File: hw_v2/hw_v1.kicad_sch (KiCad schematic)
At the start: 54 parts, among them J16 47352-1001, J8 USB_B, J9 Tag connect, SW1 SW_Push, SW2 SW_Push, U13 STM32F407VGTx, U14 TJA1051T-3, U15 25Q16, U16 REF3033, U17 SRV05-4, Y1 32.768kHz, Y2 25MHz

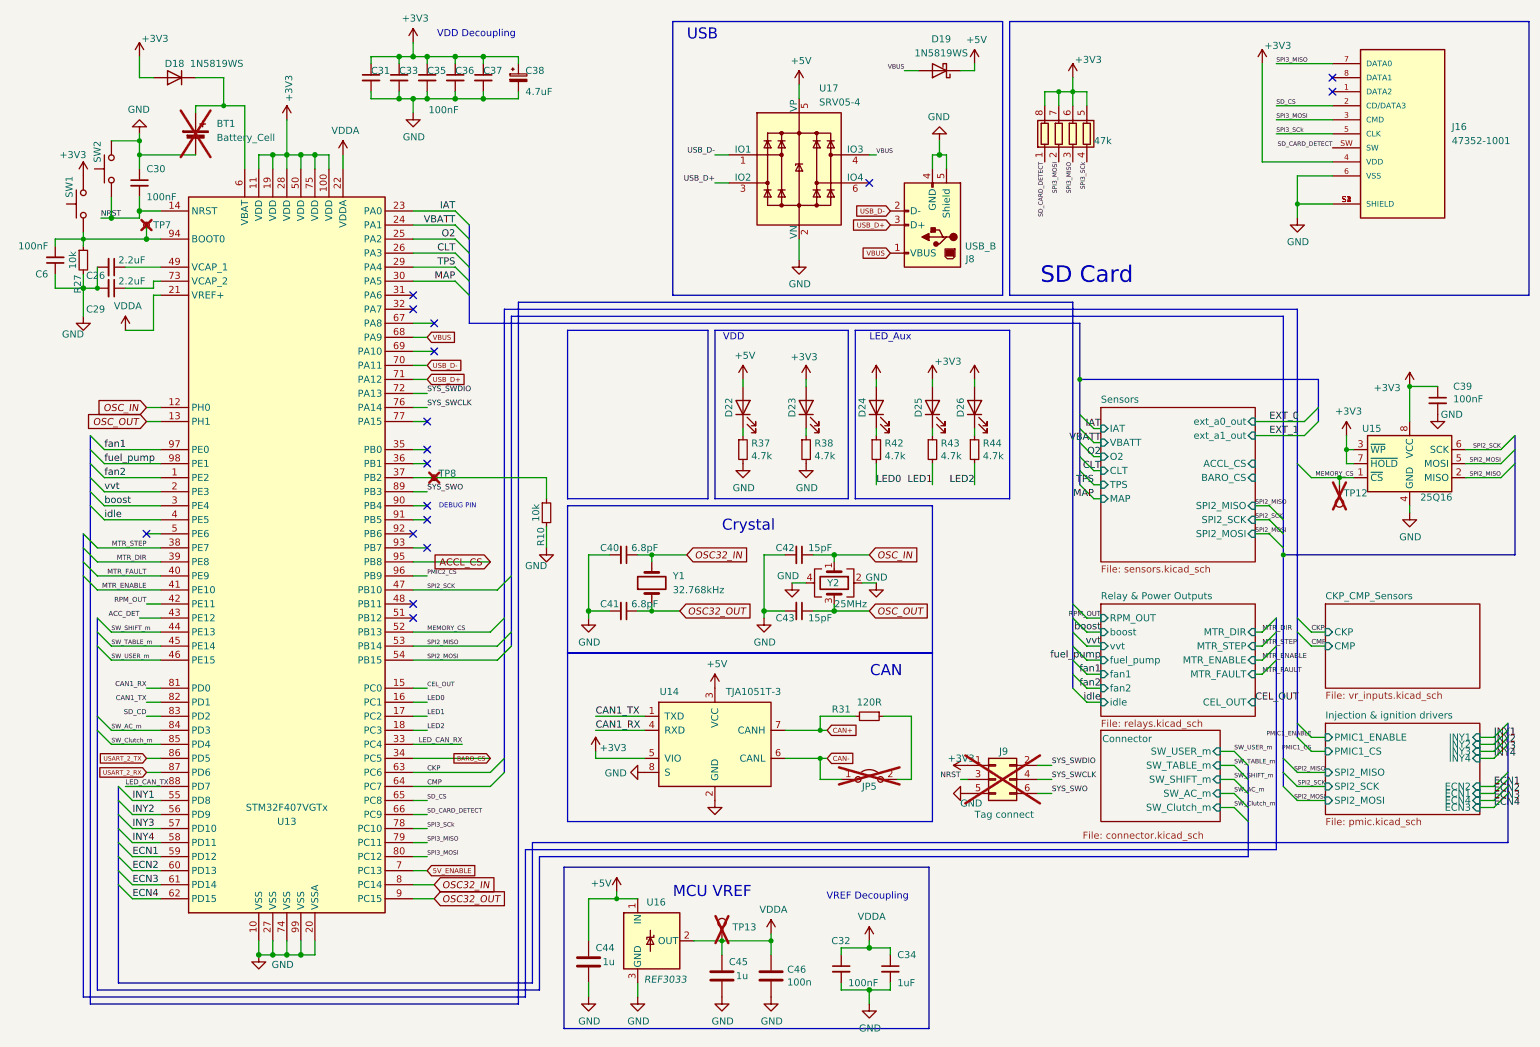
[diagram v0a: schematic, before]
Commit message: planito mas catolico
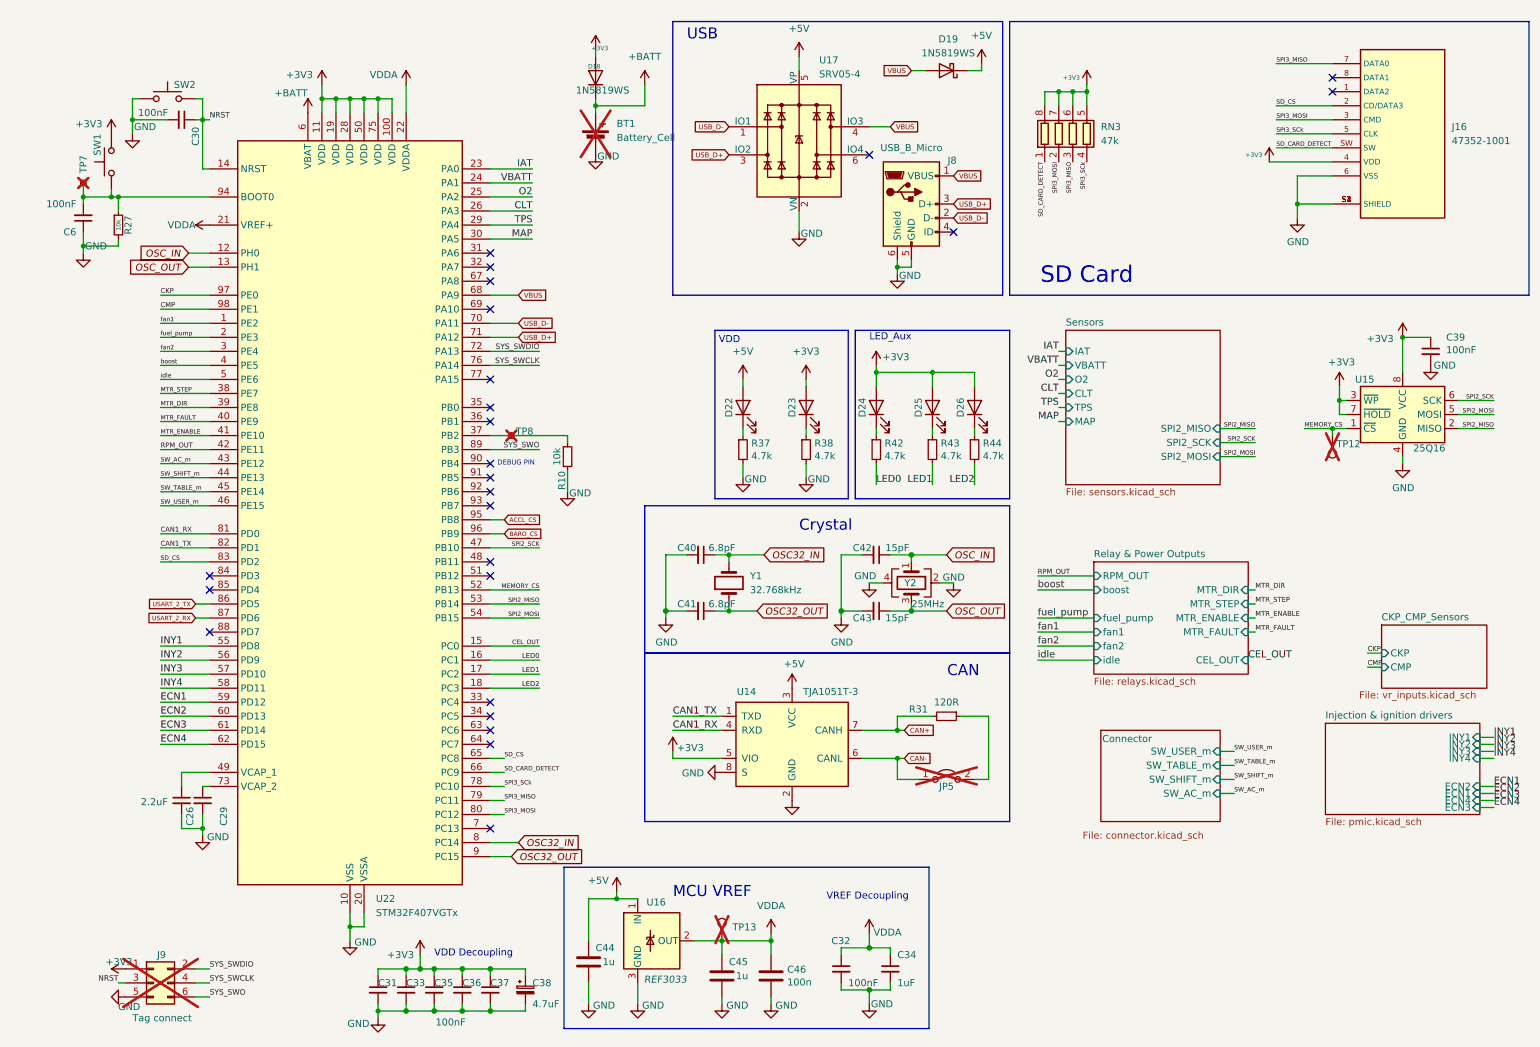
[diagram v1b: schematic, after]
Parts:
- removed J8: USB_B, Connector_USB:USB_Mini-B_Tensility_54-00023_Vertical, symbol STM32F_rev3-rescue:USB_B-Connector
- removed U13: STM32F407VGTx, Package_QFP:LQFP-100_14x14mm_P0.5mm, symbol MCU_ST_STM32F4:STM32F407VGTx
- added J8: USB_B_Micro, Connector_USB:USB_Mini-B_Tensility_54-00023_Vertical, symbol Connector:USB_B_Micro
- added U22: STM32F407VGTx, Package_QFP:LQFP-100_14x14mm_P0.5mm, symbol MCU_ST_STM32F4:STM32F407VGTx
- D18: footprint Diode_SMD:D_SOD-323_HandSoldering -> Diode_SMD:D_SOD-323
- J16: footprint uEFI_v5:MOLEX_47352-1001 -> hw_v2lib:47352-1001; symbol uEFI_v5:47352-1001 -> hw_v2:47352-1001
- RN3: footprint Resistor_SMD:R_Array_Convex_4x0603 -> (none); LCSC C779384 -> (none)
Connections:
- net +3V3: now also U22.100 (VDD), U22.11 (VDD), U22.19 (VDD), U22.28 (VDD), U22.50 (VDD), U22.75 (VDD)
- net ACCL_CS: now also U22.95 (PB8)
- net BARO_CS: now also U22.96 (PB9)
- net CAN1_RX: now also U22.81 (PD0)
- net CAN1_TX: now also U22.82 (PD1)
- net CEL_OUT: now also U22.15 (PC0)
- net CKP: now also U22.97 (PE0)
- net CLT: now also U22.26 (PA3)
- net CMP: now also U22.98 (PE1)
- net ECN1: now also U22.59 (PD12)
- net ECN2: now also U22.60 (PD13)
- net ECN3: now also U22.61 (PD14)
- net ECN4: now also U22.62 (PD15)
- net GND: now also C30.2, SW2.1, J8.5 (GND), J8.6 (Shield), U22.10 (VSS), U22.20 (VSSA), U22.27 (VSS), U22.74 (VSS), U22.99 (VSS); no longer C30.1, SW2.2
- net IAT: now also U22.23 (PA0)
- net INY1: now also U22.55 (PD8)
- net INY2: now also U22.56 (PD9)
- net INY3: now also U22.57 (PD10)
- net INY4: now also U22.58 (PD11)
- net LED0: now also U22.16 (PC1)
- net LED1: now also U22.17 (PC2)
- net LED2: now also U22.18 (PC3)
- net MAP: now also U22.30 (PA5)
- net MEMORY_CS: now also U22.52 (PB13)
- net MTR_DIR: now also U22.39 (PE8)
- net MTR_ENABLE: now also U22.41 (PE10)
- net MTR_FAULT: now also U22.40 (PE9)
- net MTR_STEP: now also U22.38 (PE7)
- net NRST: now also C30.1, SW2.2, U22.14 (NRST); no longer C30.2, SW2.1
- net O2: now also U22.25 (PA2)
- net OSC32_IN: now also U22.8 (PC14)
- net OSC32_OUT: now also U22.9 (PC15)
- net OSC_IN: now also U22.12 (PH0)
- net OSC_OUT: now also U22.13 (PH1)
- net RPM_OUT: now also U22.42 (PE11)
- net SD_CARD_DETECT: now also U22.66 (PC9)
- net SD_CS: now also U22.65 (PC8), U22.83 (PD2)
- net SPI2_MISO: now also U22.53 (PB14)
- net SPI2_MOSI: now also U22.54 (PB15)
- net SPI2_SCK: now also U22.47 (PB10)
- net SPI3_MISO: now also U22.79 (PC11)
- net SPI3_MOSI: now also U22.80 (PC12)
- net SPI3_SCk: now also U22.78 (PC10)
- net SW_AC_m: now also U22.43 (PE12)
- net SW_SHIFT_m: now also U22.44 (PE13)
- net SW_TABLE_m: now also U22.45 (PE14)
- net SW_USER_m: now also U22.46 (PE15)
- net SYS_SWCLK: now also U22.76 (PA14)
- net SYS_SWDIO: now also U22.72 (PA13)
- net SYS_SWO: now also U22.89 (PB3)
- net TPS: now also U22.29 (PA4)
- net USART_2_RX: now also U22.87 (PD6)
- net USART_2_TX: now also U22.86 (PD5)
- net USB_D+: now also J8.3 (D+), U22.71 (PA12)
- net USB_D-: now also J8.2 (D-), U22.70 (PA11)
- net VBATT: now also U22.24 (PA1)
- net VBUS: now also J8.1 (VBUS), U22.68 (PA9)
- net VDDA: now also U22.21 (VREF+), U22.22 (VDDA)
- net boost: now also U22.4 (PE5)
- net fan1: now also U22.1 (PE2)
- net fan2: now also U22.3 (PE4)
- net fuel_pump: now also U22.2 (PE3)
- net idle: now also U22.5 (PE6)
- net at C26.1: now also U22.49 (VCAP_1)
- net at C29.1: now also U22.73 (VCAP_2)
- net at R10.1, TP8.1: now also U22.37 (PB2)
- net +BATT: now reaches BT1.1 (+), D18.1 (K)
- net +BATT: now also U22.6 (VBAT)
- net at C6.2, R27.1, SW1.1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: now also U22.94 (BOOT0)
- no-connect marks 17 -> 25
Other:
- sheet Connector ports: added none; removed SW_Clutch_m
- sheet Injection & ignition drivers ports: added none; removed PMIC1_CS, PMIC1_ENABLE, SPI2_MISO, SPI2_MOSI, SPI2_SCK
- sheet Relay & Power Outputs ports: added none; removed vvt
- sheet Sensors ports: added none; removed ACCL_CS, BARO_CS, ext_a0_out, ext_a1_out
- moved on the sheet: BT1, C26, C29, C30, C31, C33, C35, C36, C37, C38, C39, C40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

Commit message: wip CKP/CMP
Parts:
- RN3: footprint (none) -> Resistor_SMD:R_Array_Convex_4x0603
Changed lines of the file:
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@@
 (kicad_sch
-	(version 20241004)
+	(version 20241209)
 	(generator "eeschema")
 	(generator_version "8.99")
@@
 			)
 		)
-		(property "Footprint" ""
+		(property "Footprint" "Resistor_SMD:R_Array_Convex_4x0603"
 			(at 207.645 34.29 90)
 			(effects
